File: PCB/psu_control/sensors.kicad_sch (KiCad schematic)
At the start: 30 parts, among them J11 Light Sensor Front, J12 Light Sensor Left, J13 Light Sensor Back, J14 Light Sensor Right, SW2 BUTTON, SW3 BUTTON, SW4 BUTTON, SW5 BUTTON, SW6 BUTTON, U5 74HC14

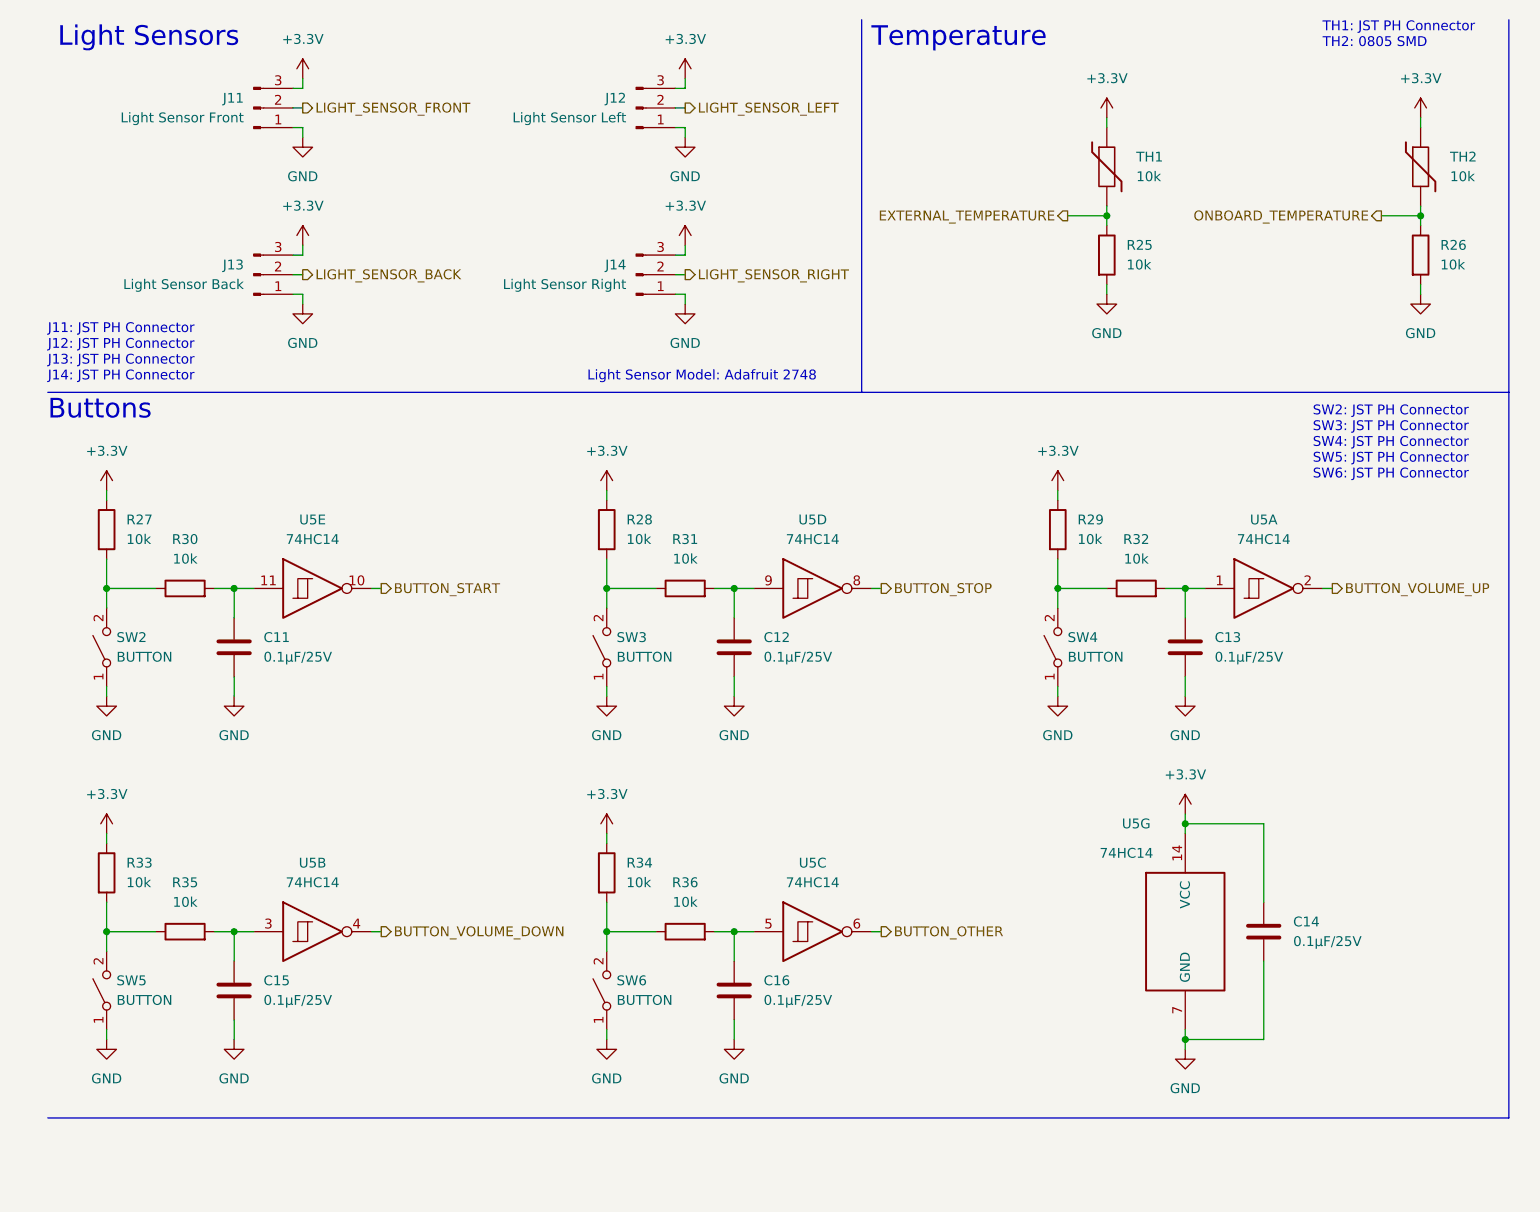
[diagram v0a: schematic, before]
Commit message: Fix PCBs.
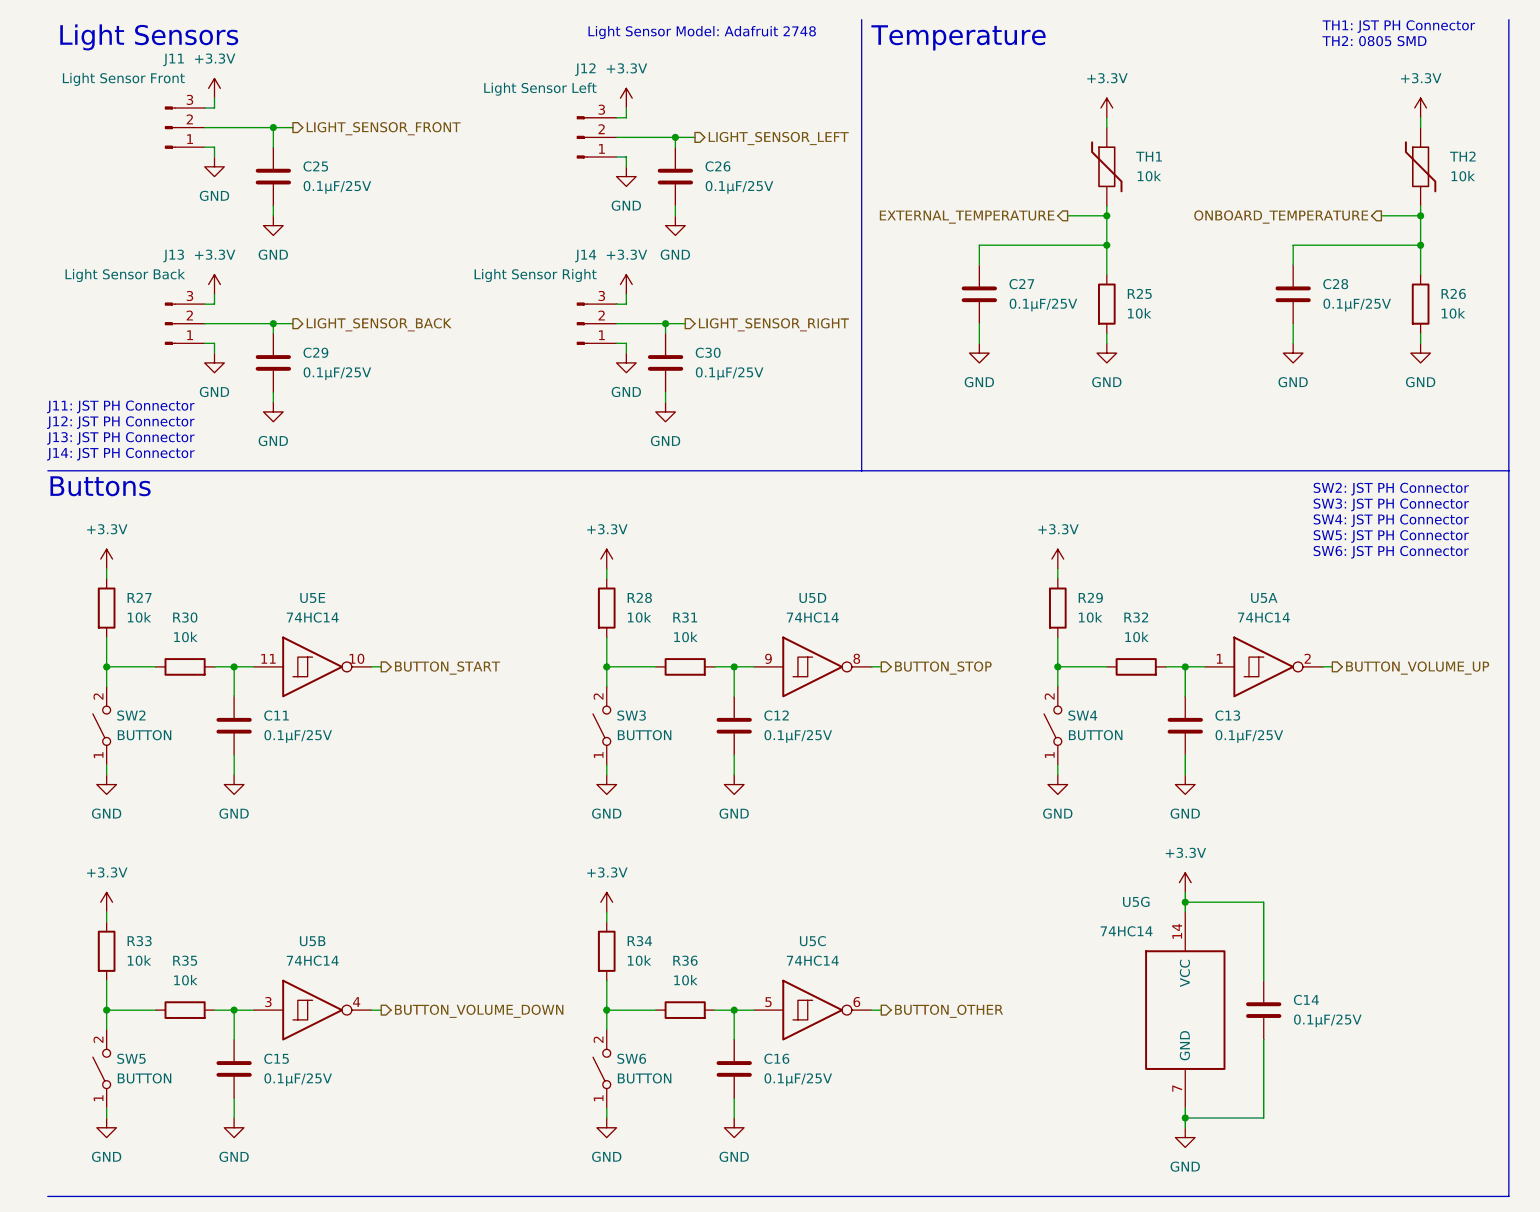
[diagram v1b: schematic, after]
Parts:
- added C25, C26, C27, C28, C29, C30: 0.1µF/25V, Capacitor_SMD:C_0805_2012Metric, symbol Device:C
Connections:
- net EXTERNAL_TEMPERATURE: now also C27.1
- net GND: now also C25.2, C26.2, C27.2, C28.2, C29.2, C30.2
- net LIGHT_SENSOR_BACK: now also C29.1
- net LIGHT_SENSOR_FRONT: now also C25.1
- net LIGHT_SENSOR_LEFT: now also C26.1
- net LIGHT_SENSOR_RIGHT: now also C30.1
- net ONBOARD_TEMPERATURE: now also C28.1
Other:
- moved on the sheet: C11, C12, C13, C14, C15, C16, J11, J12, J13, J14, R25, R26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
